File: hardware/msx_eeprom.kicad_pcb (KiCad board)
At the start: 2 copper layers, 102.8 x 65.4 mm, 103 parts, among them J1 Conn_02x07_Odd_Even, P1 MSX_CONNECTOR, U1 AT28C256-15PU

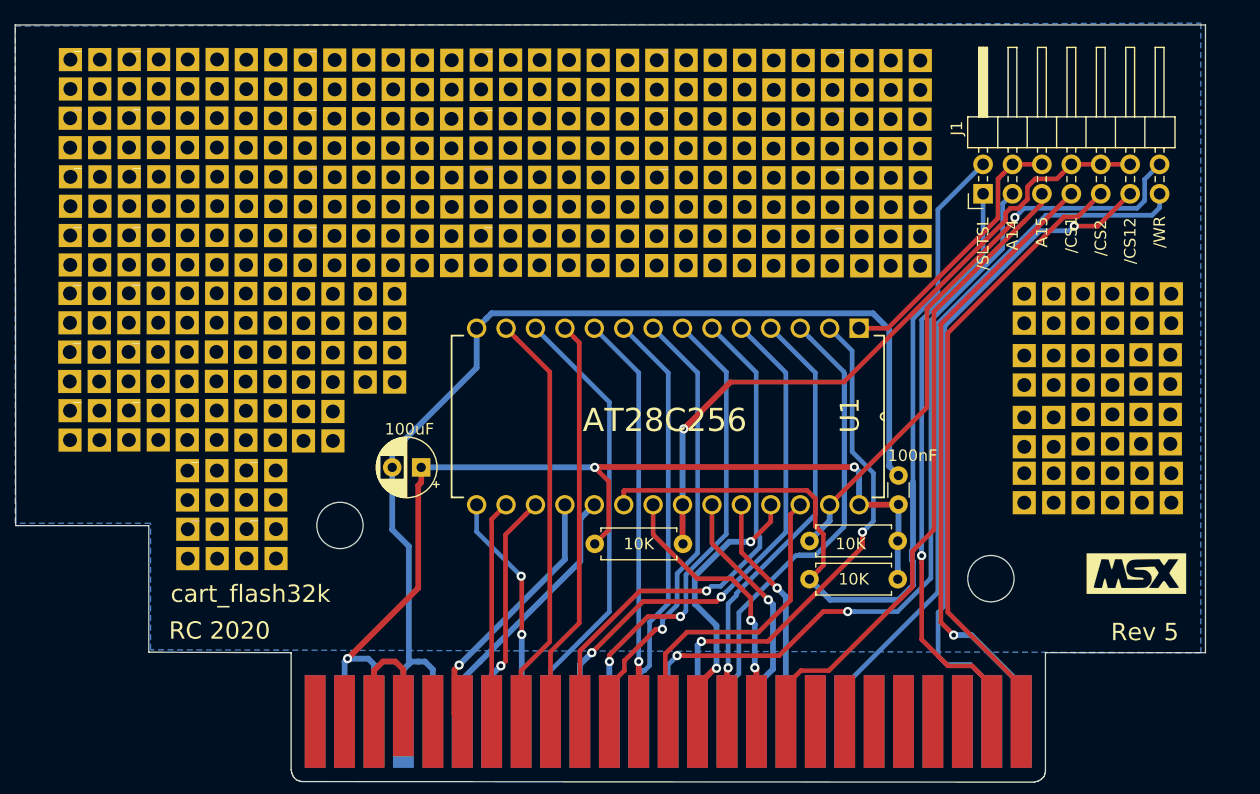
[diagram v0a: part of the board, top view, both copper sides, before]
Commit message: Imported in Kicad6
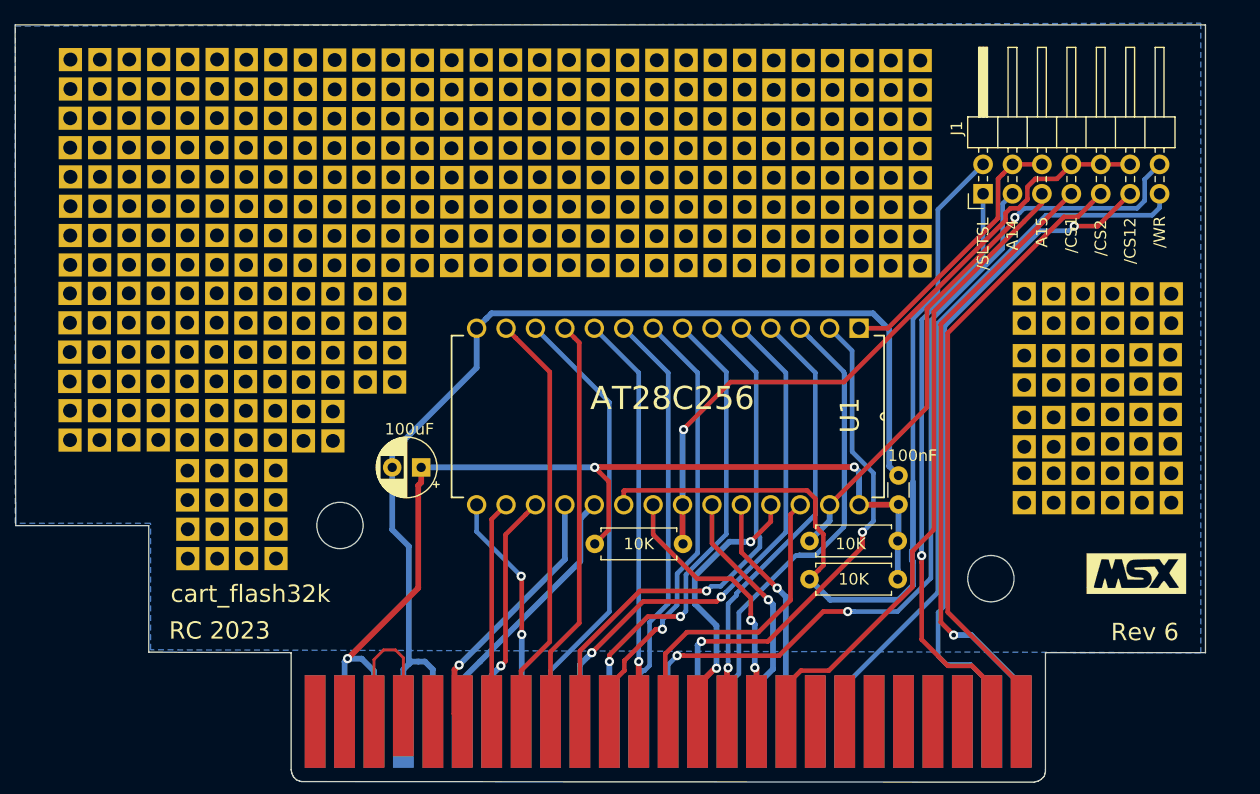
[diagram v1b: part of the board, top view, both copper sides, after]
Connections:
- P1 pad 10: Net-(P1-Pad10) -> unconnected-(P1-Pad10)
- P1 pad 11: Net-(P1-Pad11) -> unconnected-(P1-Pad11)
- P1 pad 12: Net-(P1-Pad12) -> unconnected-(P1-Pad12)
- P1 pad 15: Net-(P1-Pad15) -> unconnected-(P1-Pad15)
- P1 pad 16: Net-(P1-Pad16) -> unconnected-(P1-Pad16)
- P1 pad 42: Net-(P1-Pad42) -> unconnected-(P1-Pad42)
- P1 pad 48: Net-(P1-Pad48) -> unconnected-(P1-Pad48)
- P1 pad 49: Net-(P1-Pad49) -> unconnected-(P1-Pad49)
- P1 pad 5: Net-(P1-Pad5) -> unconnected-(P1-Pad5)
- P1 pad 50: Net-(P1-Pad50) -> unconnected-(P1-Pad50)
- P1 pad 6: Net-(P1-Pad6) -> unconnected-(P1-Pad6)
- P1 pad 7: Net-(P1-Pad7) -> unconnected-(P1-Pad7)
- P1 pad 8: Net-(P1-Pad8) -> unconnected-(P1-Pad8)
- P1 pad 9: Net-(P1-Pad9) -> unconnected-(P1-Pad9)
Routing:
- net A13: track 27.3 -> 30.7 mm
- net A14: track 69.9 -> 66.8 mm
- net Net-(P1-Pad44): track 11.5 -> 13.5 mm
- net mem_oe: track 59.6 -> 58.9 mm
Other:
- net class Default removed
- board text added: "RC 2023"
- board text added: "Rev 6"
- board text removed: "RC 2020"
- board text removed: "Rev 5"
